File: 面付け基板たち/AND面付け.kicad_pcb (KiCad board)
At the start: 2 copper layers, 99.1 x 53.3 mm, 63 parts, among them J1 Conn_01x02, J2 Conn_01x02, J3 Conn_01x02

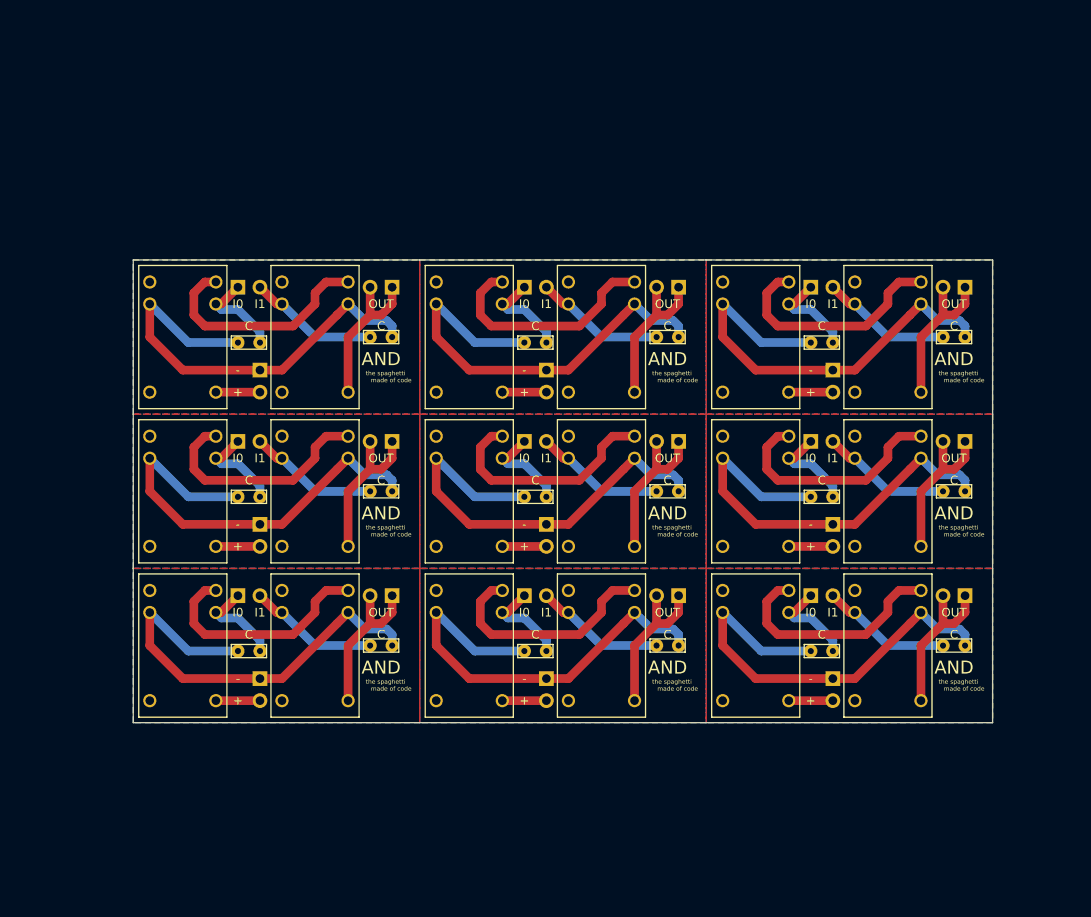
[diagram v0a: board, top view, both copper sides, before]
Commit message: Add files via upload
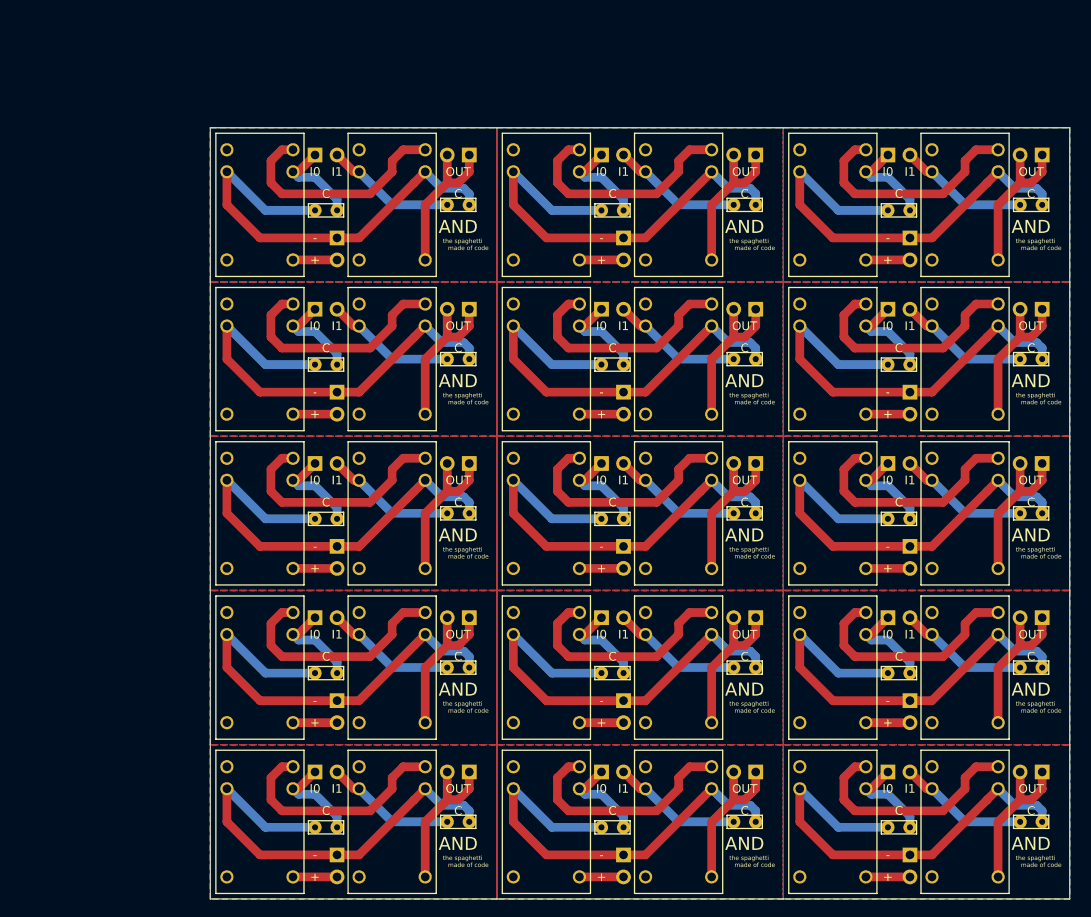
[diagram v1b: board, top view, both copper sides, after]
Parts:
- removed the C1 at (142.2, 113.7)
- removed the C1 at (109.2, 113.7)
- removed the C1 at (76.2, 113.7)
- removed the C1 at (142.2, 95.9)
- removed the C1 at (109.2, 95.9)
- removed the C1 at (76.2, 95.9)
- removed the C1 at (142.2, 78.1)
- removed the C1 at (109.2, 78.1)
- removed the C2 at (157.5, 113.0)
- removed the C2 at (124.5, 113.0)
- removed the C2 at (91.4, 113.0)
- removed the C2 at (157.5, 95.2)
- removed the C2 at (124.5, 95.2)
- removed the C2 at (91.4, 95.2)
- removed the C2 at (157.5, 77.5)
- removed the C2 at (124.5, 77.5)
- removed the J1 at (139.7, 107.3)
- removed the J1 at (106.7, 107.3)
- removed the J1 at (73.7, 107.3)
- removed the J1 at (139.7, 89.5)
- removed the J1 at (106.7, 89.5)
- removed the J1 at (73.7, 89.5)
- removed the J1 at (139.7, 71.7)
- removed the J1 at (106.7, 71.7)
- removed the J2 at (142.2, 116.8)
- removed the J2 at (109.2, 116.8)
- removed the J2 at (76.2, 116.8)
- removed the J2 at (142.2, 99.1)
- removed the J2 at (109.2, 99.1)
- removed the J2 at (76.2, 99.1)
- removed the J2 at (142.2, 81.3)
- removed the J2 at (109.2, 81.3)
- removed the J3 at (157.5, 107.3)
- removed the J3 at (124.5, 107.3)
- removed the J3 at (91.4, 107.3)
- removed the J3 at (157.5, 89.5)
- removed the J3 at (124.5, 89.5)
- removed the J3 at (91.4, 89.5)
- removed the J3 at (157.5, 71.7)
- removed the J3 at (124.5, 71.7)
- removed the SPDT1 at (134.6, 111.8)
- removed the SPDT1 at (101.6, 111.8)
- removed the SPDT1 at (68.6, 111.8)
- removed the SPDT1 at (134.6, 94.0)
- removed the SPDT1 at (101.6, 94.0)
- removed the SPDT1 at (68.6, 94.0)
- removed the SPDT1 at (134.6, 76.2)
- removed the SPDT1 at (101.6, 76.2)
- removed the SPDT2 at (149.9, 111.8)
- removed the SPDT2 at (116.8, 111.8)
- removed the SPDT2 at (83.8, 111.8)
- removed the SPDT2 at (149.9, 94.0)
- removed the SPDT2 at (116.8, 94.0)
- removed the SPDT2 at (83.8, 94.0)
- removed the SPDT2 at (149.9, 76.2)
- removed the SPDT2 at (116.8, 76.2)
- added C1: C, MiyakeFootprintLib:Condensor, F.Cu at (151.1, 134.0)
- added C1: C, MiyakeFootprintLib:Condensor, F.Cu at (151.1, 80.6)
- added C1: C, MiyakeFootprintLib:Condensor, F.Cu at (118.1, 80.6)
- added C1: C, MiyakeFootprintLib:Condensor, F.Cu at (85.1, 80.6)
- added C1: C, MiyakeFootprintLib:Condensor, F.Cu at (151.1, 62.9)
- added C1: C, MiyakeFootprintLib:Condensor, F.Cu at (118.1, 62.9)
- added C1: C, MiyakeFootprintLib:Condensor, F.Cu at (118.1, 134.0)
- added C1: C, MiyakeFootprintLib:Condensor, F.Cu at (85.1, 134.0)
- added C1: C, MiyakeFootprintLib:Condensor, F.Cu at (151.1, 116.2)
- added C1: C, MiyakeFootprintLib:Condensor, F.Cu at (118.1, 116.2)
- added C1: C, MiyakeFootprintLib:Condensor, F.Cu at (85.1, 116.2)
- added C1: C, MiyakeFootprintLib:Condensor, F.Cu at (151.1, 98.4)
- added C1: C, MiyakeFootprintLib:Condensor, F.Cu at (118.1, 98.4)
- added C1: C, MiyakeFootprintLib:Condensor, F.Cu at (85.1, 98.4)
- added C2: C, MiyakeFootprintLib:Condensor, F.Cu at (166.4, 133.3)
- added C2: C, MiyakeFootprintLib:Condensor, F.Cu at (166.4, 80.0)
- added C2: C, MiyakeFootprintLib:Condensor, F.Cu at (133.3, 80.0)
- added C2: C, MiyakeFootprintLib:Condensor, F.Cu at (100.3, 80.0)
- added C2: C, MiyakeFootprintLib:Condensor, F.Cu at (166.4, 62.2)
- added C2: C, MiyakeFootprintLib:Condensor, F.Cu at (133.3, 62.2)
- added C2: C, MiyakeFootprintLib:Condensor, F.Cu at (133.3, 133.3)
- added C2: C, MiyakeFootprintLib:Condensor, F.Cu at (100.3, 133.3)
- added C2: C, MiyakeFootprintLib:Condensor, F.Cu at (166.4, 115.6)
- added C2: C, MiyakeFootprintLib:Condensor, F.Cu at (133.3, 115.6)
- added C2: C, MiyakeFootprintLib:Condensor, F.Cu at (100.3, 115.6)
- added C2: C, MiyakeFootprintLib:Condensor, F.Cu at (166.4, 97.8)
- added C2: C, MiyakeFootprintLib:Condensor, F.Cu at (133.3, 97.8)
- added C2: C, MiyakeFootprintLib:Condensor, F.Cu at (100.3, 97.8)
- added J1: Conn_01x02, Connector_PinHeader_2.54mm:PinHeader_1x02_P2.54mm_Vertical, B.Cu at (148.6, 127.6)
- added J1: Conn_01x02, Connector_PinHeader_2.54mm:PinHeader_1x02_P2.54mm_Vertical, B.Cu at (148.6, 74.3)
- added J1: Conn_01x02, Connector_PinHeader_2.54mm:PinHeader_1x02_P2.54mm_Vertical, B.Cu at (115.6, 74.3)
- added J1: Conn_01x02, Connector_PinHeader_2.54mm:PinHeader_1x02_P2.54mm_Vertical, B.Cu at (82.5, 74.3)
- added J1: Conn_01x02, Connector_PinHeader_2.54mm:PinHeader_1x02_P2.54mm_Vertical, B.Cu at (148.6, 56.5)
- added J1: Conn_01x02, Connector_PinHeader_2.54mm:PinHeader_1x02_P2.54mm_Vertical, B.Cu at (115.6, 56.5)
- added J1: Conn_01x02, Connector_PinHeader_2.54mm:PinHeader_1x02_P2.54mm_Vertical, B.Cu at (115.6, 127.6)
- added J1: Conn_01x02, Connector_PinHeader_2.54mm:PinHeader_1x02_P2.54mm_Vertical, B.Cu at (82.5, 127.6)
- added J1: Conn_01x02, Connector_PinHeader_2.54mm:PinHeader_1x02_P2.54mm_Vertical, B.Cu at (148.6, 109.8)
- added J1: Conn_01x02, Connector_PinHeader_2.54mm:PinHeader_1x02_P2.54mm_Vertical, B.Cu at (115.6, 109.8)
- added J1: Conn_01x02, Connector_PinHeader_2.54mm:PinHeader_1x02_P2.54mm_Vertical, B.Cu at (82.5, 109.8)
- added J1: Conn_01x02, Connector_PinHeader_2.54mm:PinHeader_1x02_P2.54mm_Vertical, B.Cu at (148.6, 92.0)
- added J1: Conn_01x02, Connector_PinHeader_2.54mm:PinHeader_1x02_P2.54mm_Vertical, B.Cu at (115.6, 92.0)
- added J1: Conn_01x02, Connector_PinHeader_2.54mm:PinHeader_1x02_P2.54mm_Vertical, B.Cu at (82.5, 92.0)
- added J2: Conn_01x02, Connector_PinHeader_2.54mm:PinHeader_1x02_P2.54mm_Vertical, B.Cu at (151.1, 137.2)
- added J2: Conn_01x02, Connector_PinHeader_2.54mm:PinHeader_1x02_P2.54mm_Vertical, B.Cu at (151.1, 83.8)
- added J2: Conn_01x02, Connector_PinHeader_2.54mm:PinHeader_1x02_P2.54mm_Vertical, B.Cu at (118.1, 83.8)
- added J2: Conn_01x02, Connector_PinHeader_2.54mm:PinHeader_1x02_P2.54mm_Vertical, B.Cu at (85.1, 83.8)
- added J2: Conn_01x02, Connector_PinHeader_2.54mm:PinHeader_1x02_P2.54mm_Vertical, B.Cu at (151.1, 66.0)
- added J2: Conn_01x02, Connector_PinHeader_2.54mm:PinHeader_1x02_P2.54mm_Vertical, B.Cu at (118.1, 66.0)
- added J2: Conn_01x02, Connector_PinHeader_2.54mm:PinHeader_1x02_P2.54mm_Vertical, B.Cu at (118.1, 137.2)
- added J2: Conn_01x02, Connector_PinHeader_2.54mm:PinHeader_1x02_P2.54mm_Vertical, B.Cu at (85.1, 137.2)
- added J2: Conn_01x02, Connector_PinHeader_2.54mm:PinHeader_1x02_P2.54mm_Vertical, B.Cu at (151.1, 119.4)
- added J2: Conn_01x02, Connector_PinHeader_2.54mm:PinHeader_1x02_P2.54mm_Vertical, B.Cu at (118.1, 119.4)
- added J2: Conn_01x02, Connector_PinHeader_2.54mm:PinHeader_1x02_P2.54mm_Vertical, B.Cu at (85.1, 119.4)
- added J2: Conn_01x02, Connector_PinHeader_2.54mm:PinHeader_1x02_P2.54mm_Vertical, B.Cu at (151.1, 101.6)
- added J2: Conn_01x02, Connector_PinHeader_2.54mm:PinHeader_1x02_P2.54mm_Vertical, B.Cu at (118.1, 101.6)
- added J2: Conn_01x02, Connector_PinHeader_2.54mm:PinHeader_1x02_P2.54mm_Vertical, B.Cu at (85.1, 101.6)
- added J3: Conn_01x02, Connector_PinHeader_2.54mm:PinHeader_1x02_P2.54mm_Vertical, B.Cu at (166.4, 127.6)
- added J3: Conn_01x02, Connector_PinHeader_2.54mm:PinHeader_1x02_P2.54mm_Vertical, B.Cu at (166.4, 74.3)
- added J3: Conn_01x02, Connector_PinHeader_2.54mm:PinHeader_1x02_P2.54mm_Vertical, B.Cu at (133.3, 74.3)
- added J3: Conn_01x02, Connector_PinHeader_2.54mm:PinHeader_1x02_P2.54mm_Vertical, B.Cu at (100.3, 74.3)
- added J3: Conn_01x02, Connector_PinHeader_2.54mm:PinHeader_1x02_P2.54mm_Vertical, B.Cu at (166.4, 56.5)
- added J3: Conn_01x02, Connector_PinHeader_2.54mm:PinHeader_1x02_P2.54mm_Vertical, B.Cu at (133.3, 56.5)
- added J3: Conn_01x02, Connector_PinHeader_2.54mm:PinHeader_1x02_P2.54mm_Vertical, B.Cu at (133.3, 127.6)
- added J3: Conn_01x02, Connector_PinHeader_2.54mm:PinHeader_1x02_P2.54mm_Vertical, B.Cu at (100.3, 127.6)
- added J3: Conn_01x02, Connector_PinHeader_2.54mm:PinHeader_1x02_P2.54mm_Vertical, B.Cu at (166.4, 109.8)
- added J3: Conn_01x02, Connector_PinHeader_2.54mm:PinHeader_1x02_P2.54mm_Vertical, B.Cu at (133.3, 109.8)
- added J3: Conn_01x02, Connector_PinHeader_2.54mm:PinHeader_1x02_P2.54mm_Vertical, B.Cu at (100.3, 109.8)
- added J3: Conn_01x02, Connector_PinHeader_2.54mm:PinHeader_1x02_P2.54mm_Vertical, B.Cu at (166.4, 92.0)
- added J3: Conn_01x02, Connector_PinHeader_2.54mm:PinHeader_1x02_P2.54mm_Vertical, B.Cu at (133.3, 92.0)
- added J3: Conn_01x02, Connector_PinHeader_2.54mm:PinHeader_1x02_P2.54mm_Vertical, B.Cu at (100.3, 92.0)
- added SPDT1: 946H-1C-24D, MiyakeFootprintLib:946H-1C-24D, F.Cu at (143.5, 132.1)
- added SPDT1: 946H-1C-24D, MiyakeFootprintLib:946H-1C-24D, F.Cu at (143.5, 78.7)
- added SPDT1: 946H-1C-24D, MiyakeFootprintLib:946H-1C-24D, F.Cu at (110.5, 78.7)
- added SPDT1: 946H-1C-24D, MiyakeFootprintLib:946H-1C-24D, F.Cu at (77.5, 78.7)
- added SPDT1: 946H-1C-24D, MiyakeFootprintLib:946H-1C-24D, F.Cu at (143.5, 61.0)
- added SPDT1: 946H-1C-24D, MiyakeFootprintLib:946H-1C-24D, F.Cu at (110.5, 61.0)
- added SPDT1: 946H-1C-24D, MiyakeFootprintLib:946H-1C-24D, F.Cu at (110.5, 132.1)
- added SPDT1: 946H-1C-24D, MiyakeFootprintLib:946H-1C-24D, F.Cu at (77.5, 132.1)
- added SPDT1: 946H-1C-24D, MiyakeFootprintLib:946H-1C-24D, F.Cu at (143.5, 114.3)
- added SPDT1: 946H-1C-24D, MiyakeFootprintLib:946H-1C-24D, F.Cu at (110.5, 114.3)
- added SPDT1: 946H-1C-24D, MiyakeFootprintLib:946H-1C-24D, F.Cu at (77.5, 114.3)
- added SPDT1: 946H-1C-24D, MiyakeFootprintLib:946H-1C-24D, F.Cu at (143.5, 96.5)
- added SPDT1: 946H-1C-24D, MiyakeFootprintLib:946H-1C-24D, F.Cu at (110.5, 96.5)
- added SPDT1: 946H-1C-24D, MiyakeFootprintLib:946H-1C-24D, F.Cu at (77.5, 96.5)
- added SPDT2: 946H-1C-24D, MiyakeFootprintLib:946H-1C-24D, F.Cu at (158.8, 132.1)
- added SPDT2: 946H-1C-24D, MiyakeFootprintLib:946H-1C-24D, F.Cu at (158.8, 78.7)
- added SPDT2: 946H-1C-24D, MiyakeFootprintLib:946H-1C-24D, F.Cu at (125.7, 78.7)
- added SPDT2: 946H-1C-24D, MiyakeFootprintLib:946H-1C-24D, F.Cu at (92.7, 78.7)
- added SPDT2: 946H-1C-24D, MiyakeFootprintLib:946H-1C-24D, F.Cu at (158.8, 61.0)
- added SPDT2: 946H-1C-24D, MiyakeFootprintLib:946H-1C-24D, F.Cu at (125.7, 61.0)
- added SPDT2: 946H-1C-24D, MiyakeFootprintLib:946H-1C-24D, F.Cu at (125.7, 132.1)
- added SPDT2: 946H-1C-24D, MiyakeFootprintLib:946H-1C-24D, F.Cu at (92.7, 132.1)
- added SPDT2: 946H-1C-24D, MiyakeFootprintLib:946H-1C-24D, F.Cu at (158.8, 114.3)
- added SPDT2: 946H-1C-24D, MiyakeFootprintLib:946H-1C-24D, F.Cu at (125.7, 114.3)
- added SPDT2: 946H-1C-24D, MiyakeFootprintLib:946H-1C-24D, F.Cu at (92.7, 114.3)
- added SPDT2: 946H-1C-24D, MiyakeFootprintLib:946H-1C-24D, F.Cu at (158.8, 96.5)
- added SPDT2: 946H-1C-24D, MiyakeFootprintLib:946H-1C-24D, F.Cu at (125.7, 96.5)
- added SPDT2: 946H-1C-24D, MiyakeFootprintLib:946H-1C-24D, F.Cu at (92.7, 96.5)
- moved C1 17.6 mm to (85.1, 62.9)
- moved C2 17.6 mm to (100.3, 62.2)
- moved J1 17.6 mm to (82.5, 56.5)
- moved J3 17.6 mm to (100.3, 56.5)
- moved SPDT1 17.6 mm to (77.5, 61.0)
- moved SPDT2 17.6 mm to (92.7, 61.0)
- moved J2 17.6 mm to (85.1, 66.0)
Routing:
- net GND: track 457.3 -> 762.1 mm
- net Net-(SPDT1-Pad2): track 240.8 -> 401.4 mm
- net Net-(J3-Pad1): track 163.4 -> 272.4 mm
- net Net-(C2-Pad2): track 135.7 -> 226.2 mm
- net Net-(C1-Pad1): track 99.1 -> 165.1 mm
- net +24V: track 45.7 -> 76.2 mm
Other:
- board size 99.1 x 53.3 mm -> 99.1 x 88.9 mm

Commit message: Add files via upload
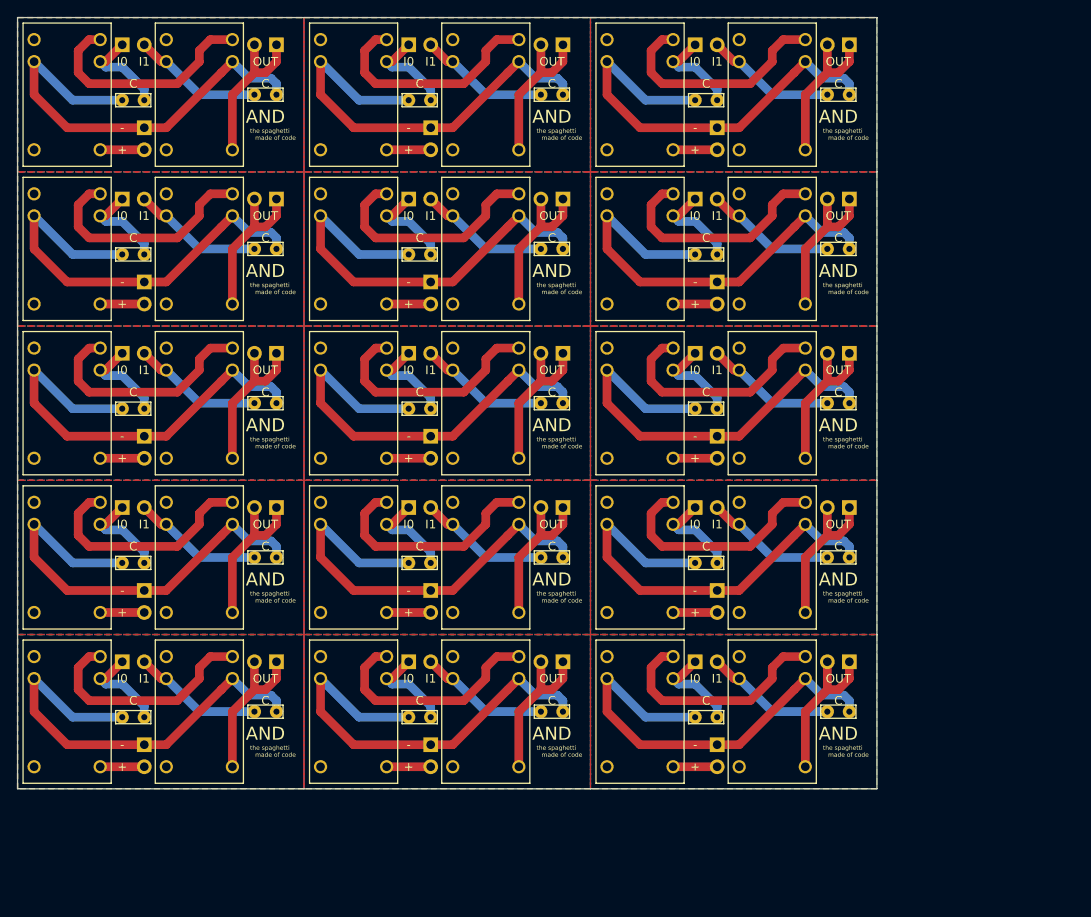
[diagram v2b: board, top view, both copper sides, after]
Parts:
- removed the C1 at (151.1, 134.0)
- removed the C1 at (151.1, 80.6)
- removed the C1 at (118.1, 80.6)
- removed the C1 at (85.1, 80.6)
- removed the C1 at (151.1, 62.9)
- removed the C1 at (118.1, 62.9)
- removed the C1 at (118.1, 134.0)
- removed the C1 at (85.1, 134.0)
- removed the C1 at (151.1, 116.2)
- removed the C1 at (118.1, 116.2)
- removed the C1 at (85.1, 116.2)
- removed the C1 at (151.1, 98.4)
- removed the C1 at (118.1, 98.4)
- removed the C1 at (85.1, 98.4)
- removed the C2 at (166.4, 133.3)
- removed the C2 at (166.4, 80.0)
- removed the C2 at (133.3, 80.0)
- removed the C2 at (100.3, 80.0)
- removed the C2 at (166.4, 62.2)
- removed the C2 at (133.3, 62.2)
- removed the C2 at (133.3, 133.3)
- removed the C2 at (100.3, 133.3)
- removed the C2 at (166.4, 115.6)
- removed the C2 at (133.3, 115.6)
- removed the C2 at (100.3, 115.6)
- removed the C2 at (166.4, 97.8)
- removed the C2 at (133.3, 97.8)
- removed the C2 at (100.3, 97.8)
- removed the J1 at (148.6, 127.6)
- removed the J1 at (148.6, 74.3)
- removed the J1 at (115.6, 74.3)
- removed the J1 at (82.5, 74.3)
- removed the J1 at (148.6, 56.5)
- removed the J1 at (115.6, 56.5)
- removed the J1 at (115.6, 127.6)
- removed the J1 at (82.5, 127.6)
- removed the J1 at (148.6, 109.8)
- removed the J1 at (115.6, 109.8)
- removed the J1 at (82.5, 109.8)
- removed the J1 at (148.6, 92.0)
- removed the J1 at (115.6, 92.0)
- removed the J1 at (82.5, 92.0)
- removed the J2 at (151.1, 137.2)
- removed the J2 at (151.1, 83.8)
- removed the J2 at (118.1, 83.8)
- removed the J2 at (85.1, 83.8)
- removed the J2 at (151.1, 66.0)
- removed the J2 at (118.1, 66.0)
- removed the J2 at (118.1, 137.2)
- removed the J2 at (85.1, 137.2)
- removed the J2 at (151.1, 119.4)
- removed the J2 at (118.1, 119.4)
- removed the J2 at (85.1, 119.4)
- removed the J2 at (151.1, 101.6)
- removed the J2 at (118.1, 101.6)
- removed the J2 at (85.1, 101.6)
- removed the J3 at (166.4, 127.6)
- removed the J3 at (166.4, 74.3)
- removed the J3 at (133.3, 74.3)
- removed the J3 at (100.3, 74.3)
- removed the J3 at (166.4, 56.5)
- removed the J3 at (133.3, 56.5)
- removed the J3 at (133.3, 127.6)
- removed the J3 at (100.3, 127.6)
- removed the J3 at (166.4, 109.8)
- removed the J3 at (133.3, 109.8)
- removed the J3 at (100.3, 109.8)
- removed the J3 at (166.4, 92.0)
- removed the J3 at (133.3, 92.0)
- removed the J3 at (100.3, 92.0)
- removed the SPDT1 at (143.5, 132.1)
- removed the SPDT1 at (143.5, 78.7)
- removed the SPDT1 at (110.5, 78.7)
- removed the SPDT1 at (77.5, 78.7)
- removed the SPDT1 at (143.5, 61.0)
- removed the SPDT1 at (110.5, 61.0)
- removed the SPDT1 at (110.5, 132.1)
- removed the SPDT1 at (77.5, 132.1)
- removed the SPDT1 at (143.5, 114.3)
- removed the SPDT1 at (110.5, 114.3)
- removed the SPDT1 at (77.5, 114.3)
- removed the SPDT1 at (143.5, 96.5)
- removed the SPDT1 at (110.5, 96.5)
- removed the SPDT1 at (77.5, 96.5)
- removed the SPDT2 at (158.8, 132.1)
- removed the SPDT2 at (158.8, 78.7)
- removed the SPDT2 at (125.7, 78.7)
- removed the SPDT2 at (92.7, 78.7)
- removed the SPDT2 at (158.8, 61.0)
- removed the SPDT2 at (125.7, 61.0)
- removed the SPDT2 at (125.7, 132.1)
- removed the SPDT2 at (92.7, 132.1)
- removed the SPDT2 at (158.8, 114.3)
- removed the SPDT2 at (125.7, 114.3)
- removed the SPDT2 at (92.7, 114.3)
- removed the SPDT2 at (158.8, 96.5)
- removed the SPDT2 at (125.7, 96.5)
- removed the SPDT2 at (92.7, 96.5)
- added C1: C, MiyakeFootprintLib:Condensor, F.Cu at (128.9, 121.3)
- added C1: C, MiyakeFootprintLib:Condensor, F.Cu at (128.9, 67.9)
- added C1: C, MiyakeFootprintLib:Condensor, F.Cu at (95.9, 67.9)
- added C1: C, MiyakeFootprintLib:Condensor, F.Cu at (62.9, 67.9)
- added C1: C, MiyakeFootprintLib:Condensor, F.Cu at (128.9, 50.2)
- added C1: C, MiyakeFootprintLib:Condensor, F.Cu at (95.9, 50.2)
- added C1: C, MiyakeFootprintLib:Condensor, F.Cu at (95.9, 121.3)
- added C1: C, MiyakeFootprintLib:Condensor, F.Cu at (62.9, 121.3)
- added C1: C, MiyakeFootprintLib:Condensor, F.Cu at (128.9, 103.5)
- added C1: C, MiyakeFootprintLib:Condensor, F.Cu at (95.9, 103.5)
- added C1: C, MiyakeFootprintLib:Condensor, F.Cu at (62.9, 103.5)
- added C1: C, MiyakeFootprintLib:Condensor, F.Cu at (128.9, 85.7)
- added C1: C, MiyakeFootprintLib:Condensor, F.Cu at (95.9, 85.7)
- added C1: C, MiyakeFootprintLib:Condensor, F.Cu at (62.9, 85.7)
- added C2: C, MiyakeFootprintLib:Condensor, F.Cu at (144.1, 120.7)
- added C2: C, MiyakeFootprintLib:Condensor, F.Cu at (144.1, 67.3)
- added C2: C, MiyakeFootprintLib:Condensor, F.Cu at (111.1, 67.3)
- added C2: C, MiyakeFootprintLib:Condensor, F.Cu at (78.1, 67.3)
- added C2: C, MiyakeFootprintLib:Condensor, F.Cu at (144.1, 49.5)
- added C2: C, MiyakeFootprintLib:Condensor, F.Cu at (111.1, 49.5)
- added C2: C, MiyakeFootprintLib:Condensor, F.Cu at (111.1, 120.7)
- added C2: C, MiyakeFootprintLib:Condensor, F.Cu at (78.1, 120.7)
- added C2: C, MiyakeFootprintLib:Condensor, F.Cu at (144.1, 102.9)
- added C2: C, MiyakeFootprintLib:Condensor, F.Cu at (111.1, 102.9)
- added C2: C, MiyakeFootprintLib:Condensor, F.Cu at (78.1, 102.9)
- added C2: C, MiyakeFootprintLib:Condensor, F.Cu at (144.1, 85.1)
- added C2: C, MiyakeFootprintLib:Condensor, F.Cu at (111.1, 85.1)
- added C2: C, MiyakeFootprintLib:Condensor, F.Cu at (78.1, 85.1)
- added J1: Conn_01x02, Connector_PinHeader_2.54mm:PinHeader_1x02_P2.54mm_Vertical, B.Cu at (126.4, 114.9)
- added J1: Conn_01x02, Connector_PinHeader_2.54mm:PinHeader_1x02_P2.54mm_Vertical, B.Cu at (126.4, 61.6)
- added J1: Conn_01x02, Connector_PinHeader_2.54mm:PinHeader_1x02_P2.54mm_Vertical, B.Cu at (93.3, 61.6)
- added J1: Conn_01x02, Connector_PinHeader_2.54mm:PinHeader_1x02_P2.54mm_Vertical, B.Cu at (60.3, 61.6)
- added J1: Conn_01x02, Connector_PinHeader_2.54mm:PinHeader_1x02_P2.54mm_Vertical, B.Cu at (126.4, 43.8)
- added J1: Conn_01x02, Connector_PinHeader_2.54mm:PinHeader_1x02_P2.54mm_Vertical, B.Cu at (93.3, 43.8)
- added J1: Conn_01x02, Connector_PinHeader_2.54mm:PinHeader_1x02_P2.54mm_Vertical, B.Cu at (93.3, 114.9)
- added J1: Conn_01x02, Connector_PinHeader_2.54mm:PinHeader_1x02_P2.54mm_Vertical, B.Cu at (60.3, 114.9)
- added J1: Conn_01x02, Connector_PinHeader_2.54mm:PinHeader_1x02_P2.54mm_Vertical, B.Cu at (126.4, 97.1)
- added J1: Conn_01x02, Connector_PinHeader_2.54mm:PinHeader_1x02_P2.54mm_Vertical, B.Cu at (93.3, 97.1)
- added J1: Conn_01x02, Connector_PinHeader_2.54mm:PinHeader_1x02_P2.54mm_Vertical, B.Cu at (60.3, 97.1)
- added J1: Conn_01x02, Connector_PinHeader_2.54mm:PinHeader_1x02_P2.54mm_Vertical, B.Cu at (126.4, 79.3)
- added J1: Conn_01x02, Connector_PinHeader_2.54mm:PinHeader_1x02_P2.54mm_Vertical, B.Cu at (93.3, 79.3)
- added J1: Conn_01x02, Connector_PinHeader_2.54mm:PinHeader_1x02_P2.54mm_Vertical, B.Cu at (60.3, 79.3)
- added J2: Conn_01x02, Connector_PinHeader_2.54mm:PinHeader_1x02_P2.54mm_Vertical, B.Cu at (128.9, 124.5)
- added J2: Conn_01x02, Connector_PinHeader_2.54mm:PinHeader_1x02_P2.54mm_Vertical, B.Cu at (128.9, 71.1)
- added J2: Conn_01x02, Connector_PinHeader_2.54mm:PinHeader_1x02_P2.54mm_Vertical, B.Cu at (95.9, 71.1)
- added J2: Conn_01x02, Connector_PinHeader_2.54mm:PinHeader_1x02_P2.54mm_Vertical, B.Cu at (62.9, 71.1)
- added J2: Conn_01x02, Connector_PinHeader_2.54mm:PinHeader_1x02_P2.54mm_Vertical, B.Cu at (128.9, 53.3)
- added J2: Conn_01x02, Connector_PinHeader_2.54mm:PinHeader_1x02_P2.54mm_Vertical, B.Cu at (95.9, 53.3)
- added J2: Conn_01x02, Connector_PinHeader_2.54mm:PinHeader_1x02_P2.54mm_Vertical, B.Cu at (95.9, 124.5)
- added J2: Conn_01x02, Connector_PinHeader_2.54mm:PinHeader_1x02_P2.54mm_Vertical, B.Cu at (62.9, 124.5)
- added J2: Conn_01x02, Connector_PinHeader_2.54mm:PinHeader_1x02_P2.54mm_Vertical, B.Cu at (128.9, 106.7)
- added J2: Conn_01x02, Connector_PinHeader_2.54mm:PinHeader_1x02_P2.54mm_Vertical, B.Cu at (95.9, 106.7)
- added J2: Conn_01x02, Connector_PinHeader_2.54mm:PinHeader_1x02_P2.54mm_Vertical, B.Cu at (62.9, 106.7)
- added J2: Conn_01x02, Connector_PinHeader_2.54mm:PinHeader_1x02_P2.54mm_Vertical, B.Cu at (128.9, 88.9)
- added J2: Conn_01x02, Connector_PinHeader_2.54mm:PinHeader_1x02_P2.54mm_Vertical, B.Cu at (95.9, 88.9)
- added J2: Conn_01x02, Connector_PinHeader_2.54mm:PinHeader_1x02_P2.54mm_Vertical, B.Cu at (62.9, 88.9)
- added J3: Conn_01x02, Connector_PinHeader_2.54mm:PinHeader_1x02_P2.54mm_Vertical, B.Cu at (144.1, 114.9)
- added J3: Conn_01x02, Connector_PinHeader_2.54mm:PinHeader_1x02_P2.54mm_Vertical, B.Cu at (144.1, 61.6)
- added J3: Conn_01x02, Connector_PinHeader_2.54mm:PinHeader_1x02_P2.54mm_Vertical, B.Cu at (111.1, 61.6)
- added J3: Conn_01x02, Connector_PinHeader_2.54mm:PinHeader_1x02_P2.54mm_Vertical, B.Cu at (78.1, 61.6)
- added J3: Conn_01x02, Connector_PinHeader_2.54mm:PinHeader_1x02_P2.54mm_Vertical, B.Cu at (144.1, 43.8)
- added J3: Conn_01x02, Connector_PinHeader_2.54mm:PinHeader_1x02_P2.54mm_Vertical, B.Cu at (111.1, 43.8)
- added J3: Conn_01x02, Connector_PinHeader_2.54mm:PinHeader_1x02_P2.54mm_Vertical, B.Cu at (111.1, 114.9)
- added J3: Conn_01x02, Connector_PinHeader_2.54mm:PinHeader_1x02_P2.54mm_Vertical, B.Cu at (78.1, 114.9)
- added J3: Conn_01x02, Connector_PinHeader_2.54mm:PinHeader_1x02_P2.54mm_Vertical, B.Cu at (144.1, 97.1)
- added J3: Conn_01x02, Connector_PinHeader_2.54mm:PinHeader_1x02_P2.54mm_Vertical, B.Cu at (111.1, 97.1)
- added J3: Conn_01x02, Connector_PinHeader_2.54mm:PinHeader_1x02_P2.54mm_Vertical, B.Cu at (78.1, 97.1)
- added J3: Conn_01x02, Connector_PinHeader_2.54mm:PinHeader_1x02_P2.54mm_Vertical, B.Cu at (144.1, 79.3)
- added J3: Conn_01x02, Connector_PinHeader_2.54mm:PinHeader_1x02_P2.54mm_Vertical, B.Cu at (111.1, 79.3)
- added J3: Conn_01x02, Connector_PinHeader_2.54mm:PinHeader_1x02_P2.54mm_Vertical, B.Cu at (78.1, 79.3)
- added SPDT1: 946H-1C-24D, MiyakeFootprintLib:946H-1C-24D, F.Cu at (121.3, 119.4)
- added SPDT1: 946H-1C-24D, MiyakeFootprintLib:946H-1C-24D, F.Cu at (121.3, 66.0)
- added SPDT1: 946H-1C-24D, MiyakeFootprintLib:946H-1C-24D, F.Cu at (88.3, 66.0)
- added SPDT1: 946H-1C-24D, MiyakeFootprintLib:946H-1C-24D, F.Cu at (55.2, 66.0)
- added SPDT1: 946H-1C-24D, MiyakeFootprintLib:946H-1C-24D, F.Cu at (121.3, 48.3)
- added SPDT1: 946H-1C-24D, MiyakeFootprintLib:946H-1C-24D, F.Cu at (88.3, 48.3)
- added SPDT1: 946H-1C-24D, MiyakeFootprintLib:946H-1C-24D, F.Cu at (88.3, 119.4)
- added SPDT1: 946H-1C-24D, MiyakeFootprintLib:946H-1C-24D, F.Cu at (55.2, 119.4)
- added SPDT1: 946H-1C-24D, MiyakeFootprintLib:946H-1C-24D, F.Cu at (121.3, 101.6)
- added SPDT1: 946H-1C-24D, MiyakeFootprintLib:946H-1C-24D, F.Cu at (88.3, 101.6)
- added SPDT1: 946H-1C-24D, MiyakeFootprintLib:946H-1C-24D, F.Cu at (55.2, 101.6)
- added SPDT1: 946H-1C-24D, MiyakeFootprintLib:946H-1C-24D, F.Cu at (121.3, 83.8)
- added SPDT1: 946H-1C-24D, MiyakeFootprintLib:946H-1C-24D, F.Cu at (88.3, 83.8)
- added SPDT1: 946H-1C-24D, MiyakeFootprintLib:946H-1C-24D, F.Cu at (55.2, 83.8)
- added SPDT2: 946H-1C-24D, MiyakeFootprintLib:946H-1C-24D, F.Cu at (136.5, 119.4)
- added SPDT2: 946H-1C-24D, MiyakeFootprintLib:946H-1C-24D, F.Cu at (136.5, 66.0)
- added SPDT2: 946H-1C-24D, MiyakeFootprintLib:946H-1C-24D, F.Cu at (103.5, 66.0)
- added SPDT2: 946H-1C-24D, MiyakeFootprintLib:946H-1C-24D, F.Cu at (70.5, 66.0)
- added SPDT2: 946H-1C-24D, MiyakeFootprintLib:946H-1C-24D, F.Cu at (136.5, 48.3)
- added SPDT2: 946H-1C-24D, MiyakeFootprintLib:946H-1C-24D, F.Cu at (103.5, 48.3)
- added SPDT2: 946H-1C-24D, MiyakeFootprintLib:946H-1C-24D, F.Cu at (103.5, 119.4)
- added SPDT2: 946H-1C-24D, MiyakeFootprintLib:946H-1C-24D, F.Cu at (70.5, 119.4)
- added SPDT2: 946H-1C-24D, MiyakeFootprintLib:946H-1C-24D, F.Cu at (136.5, 101.6)
- added SPDT2: 946H-1C-24D, MiyakeFootprintLib:946H-1C-24D, F.Cu at (103.5, 101.6)
- added SPDT2: 946H-1C-24D, MiyakeFootprintLib:946H-1C-24D, F.Cu at (70.5, 101.6)
- added SPDT2: 946H-1C-24D, MiyakeFootprintLib:946H-1C-24D, F.Cu at (136.5, 83.8)
- added SPDT2: 946H-1C-24D, MiyakeFootprintLib:946H-1C-24D, F.Cu at (103.5, 83.8)
- added SPDT2: 946H-1C-24D, MiyakeFootprintLib:946H-1C-24D, F.Cu at (70.5, 83.8)
- moved C1 25.6 mm to (62.9, 50.2)
- moved J2 25.6 mm to (62.9, 53.3)
- moved SPDT1 25.6 mm to (55.2, 48.3)
- moved SPDT2 25.6 mm to (70.5, 48.3)
- moved C2 25.6 mm to (78.1, 49.5)
- moved J1 25.6 mm to (60.3, 43.8)
- moved J3 25.6 mm to (78.1, 43.8)
